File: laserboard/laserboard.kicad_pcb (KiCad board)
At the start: 4 copper layers, 167.5 x 113.5 mm, 90 parts, among them J1 Conn_01x02, J2 USB_C_Receptacle_USB2.0_16P, J3 Conn_01x19, J4 Conn_01x19, U1 AD8656, U2 PGA112, U3 AD8655, U5 NCP1117-3.3_SOT223, U6 W25Q128JVS, U7 RP2040, Y1 ABM8-272-T3

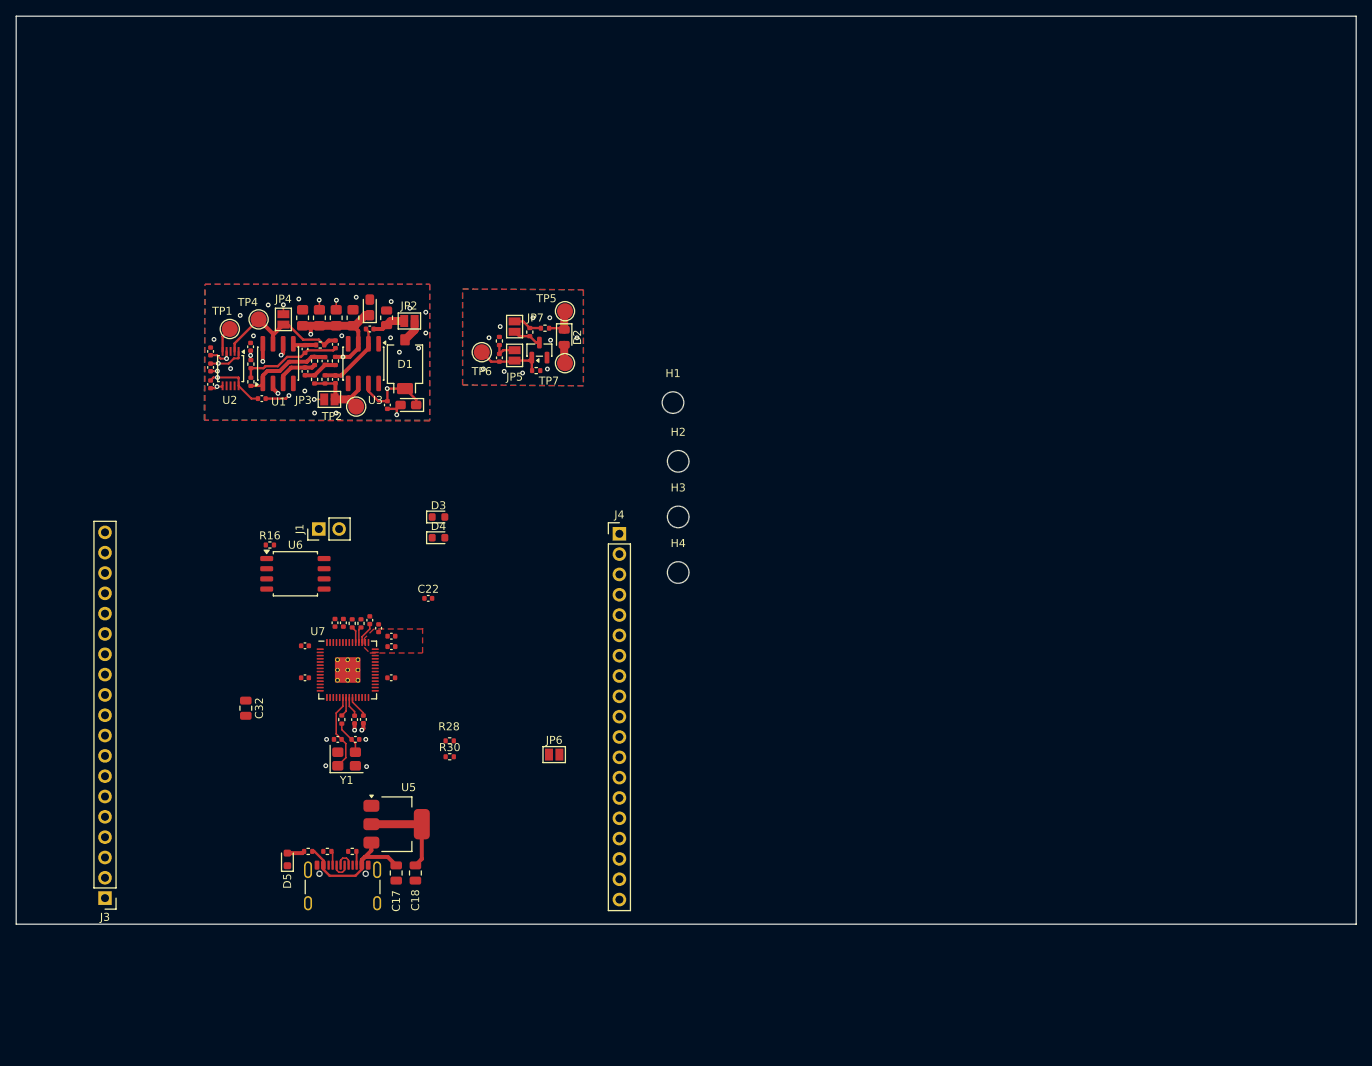
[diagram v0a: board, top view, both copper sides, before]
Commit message: PCB_prot
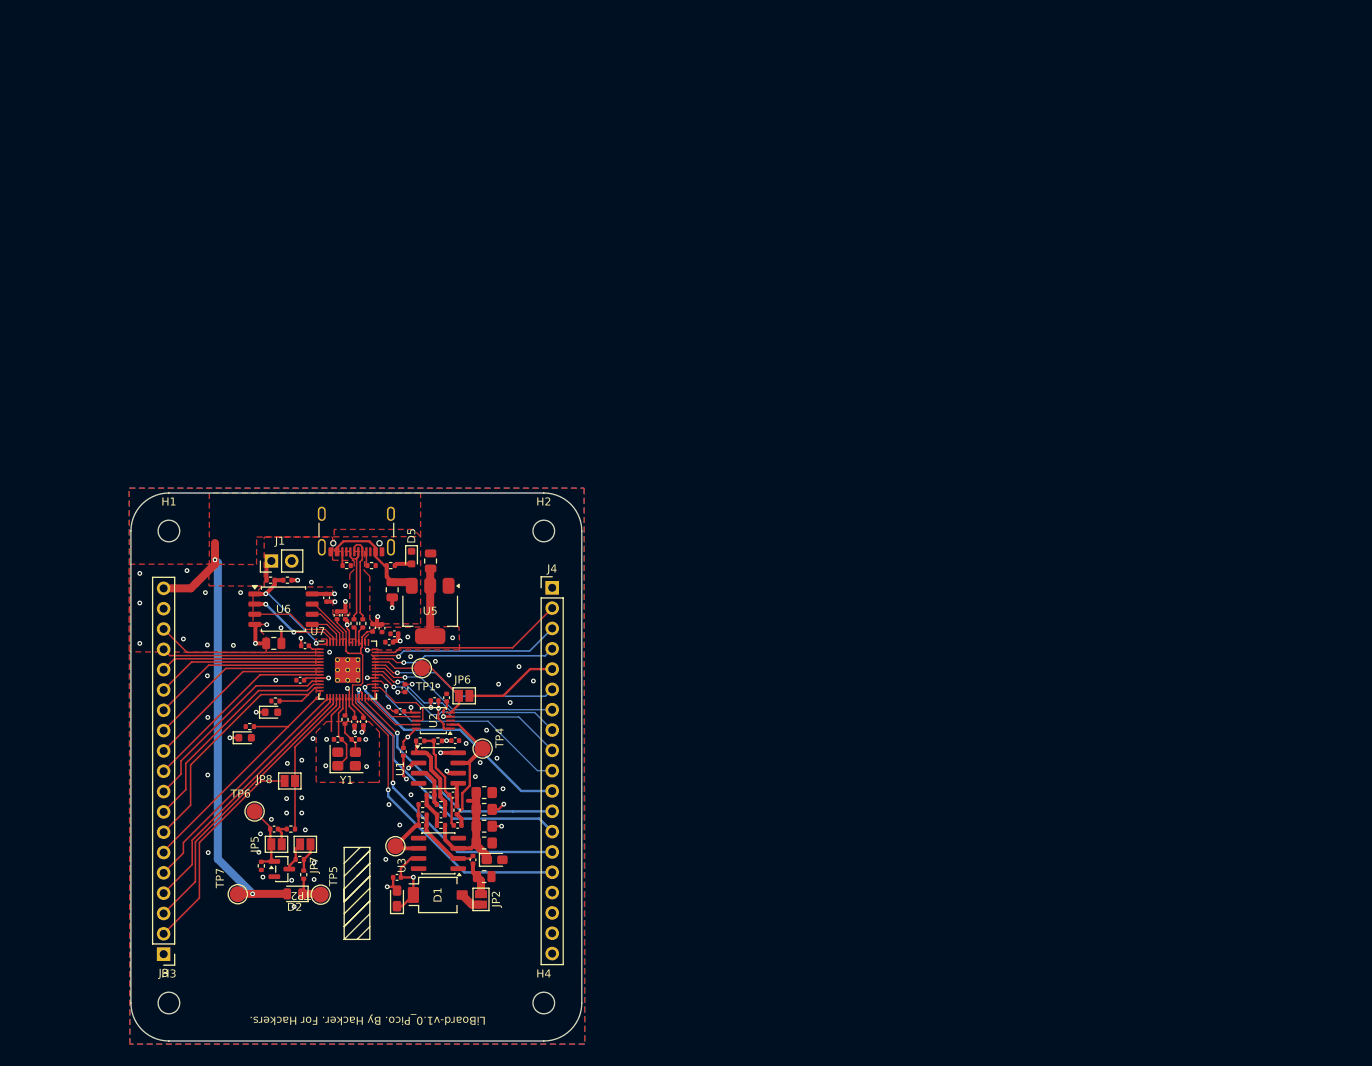
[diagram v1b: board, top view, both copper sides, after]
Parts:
- removed JP3, JP4: SolderJumper_2_Open, Jumper:SolderJumper-2_P1.3mm_Open_Pad1.0x1.5mm
- added JP8: SolderJumper_2_Open, Jumper:SolderJumper-2_P1.3mm_Open_Pad1.0x1.5mm, F.Cu at (117.2, 133.1)
- added R17: DNF, Resistor_SMD:R_0402_1005Metric, F.Cu at (116.9, 108.0)
- moved H3 88.0 mm to (102.1, 160.8)
- moved TP5 79.1 mm to (121.1, 147.3), turned to 180 degrees
- moved TP7 78.0 mm to (110.7, 147.2), turned to 180 degrees
- moved D2 77.3 mm to (117.8, 147.2), turned to 180 degrees
- moved R13 74.7 mm to (118.9, 144.8), turned to -90 degrees
- moved JP2 72.9 mm to (141.1, 147.9), turned to -90 degrees
- moved N-MOS1 72.4 mm to (116.2, 144.1), turned to 0 degrees
- moved R27 71.9 mm to (118.5, 142.9), turned to 0 degrees
- moved R29 70.9 mm to (141.5, 145.1), turned to 180 degrees
- moved R15 70.8 mm to (113.6, 143.7), turned to 90 degrees
- moved C33 70.8 mm to (142.8, 142.9), turned to 0 degrees
- moved JP7 69.8 mm to (119.1, 141.0), turned to 180 degrees
- moved JP5 68.0 mm to (115.5, 141.0), turned to 0 degrees
- moved R26 67.7 mm to (141.5, 140.8), turned to 0 degrees
- moved C20 67.6 mm to (140.1, 142.9), turned to -90 degrees
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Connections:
- J4 pad 12: /Didital/GPIO19 -> /Didital/GPIO16
- J4 pad 13: /Didital/GPIO18 -> /Didital/RUN
- J4 pad 14: /Didital/GPIO17 -> /Didital/SWD
- J4 pad 15: /Didital/GPIO16 -> /Didital/SWCLK
- J4 pad 16: /Didital/RUN -> GND
- J4 pad 17: /Didital/SWD -> GND
- J4 pad 18: /Didital/SWCLK -> GND
- R14 pad 1: /Didital/GPIO0 -> /Didital/TX_D_IN
- R28 pad 2: /Didital/GPIO25 -> /Didital/GPIO10
- R30 pad 2: /Didital/GPIO24 -> /Didital/GPIO11
- U7 pad 18: /Didital/GPIO15 -> /Didital/TX_D_IN
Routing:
- net +5V: track 19.5 -> 74.2 mm, vias 0 -> 2
- net /Didital/SWCLK: track 0.00 -> 38.5 mm, vias 0 -> 1
- net /Didital/SWD: track 0.00 -> 36.3 mm, vias 0 -> 1
- net /Didital/GPIO14: track 0.00 -> 35.8 mm
- net /Didital/RUN: track 0.00 -> 35.3 mm, vias 0 -> 1
- net /Didital/GPIO10: track 0.00 -> 33.9 mm
- net /Didital/GPIO13: track 0.00 -> 33.1 mm
- net /Didital/GPIO11: track 0.00 -> 32.6 mm
- net /Didital/GPIO16: track 0.00 -> 30.6 mm, vias 0 -> 1
- net /Didital/GPIO20: track 0.00 -> 30.4 mm, vias 0 -> 1
- net /Didital/GPIO12: track 0.00 -> 30.4 mm
- net /Didital/GPIO9: track 0.00 -> 28.1 mm
- net /Didital/GPIO21: track 0.00 -> 27.5 mm, vias 0 -> 1
- net /Didital/GPIO15: track 0.00 -> 27.1 mm
- net /Didital/GPIO22: track 0.00 -> 26.3 mm, vias 0 -> 1
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- added copper zone on F.Cu, net +5V
- removed copper zone on In2.Cu, net GND
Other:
- board size 167.5 x 113.5 mm -> 56.4 x 68.5 mm
- board text added: "LiBoard-v1.0_Pico. By Hacker. For Hackers."

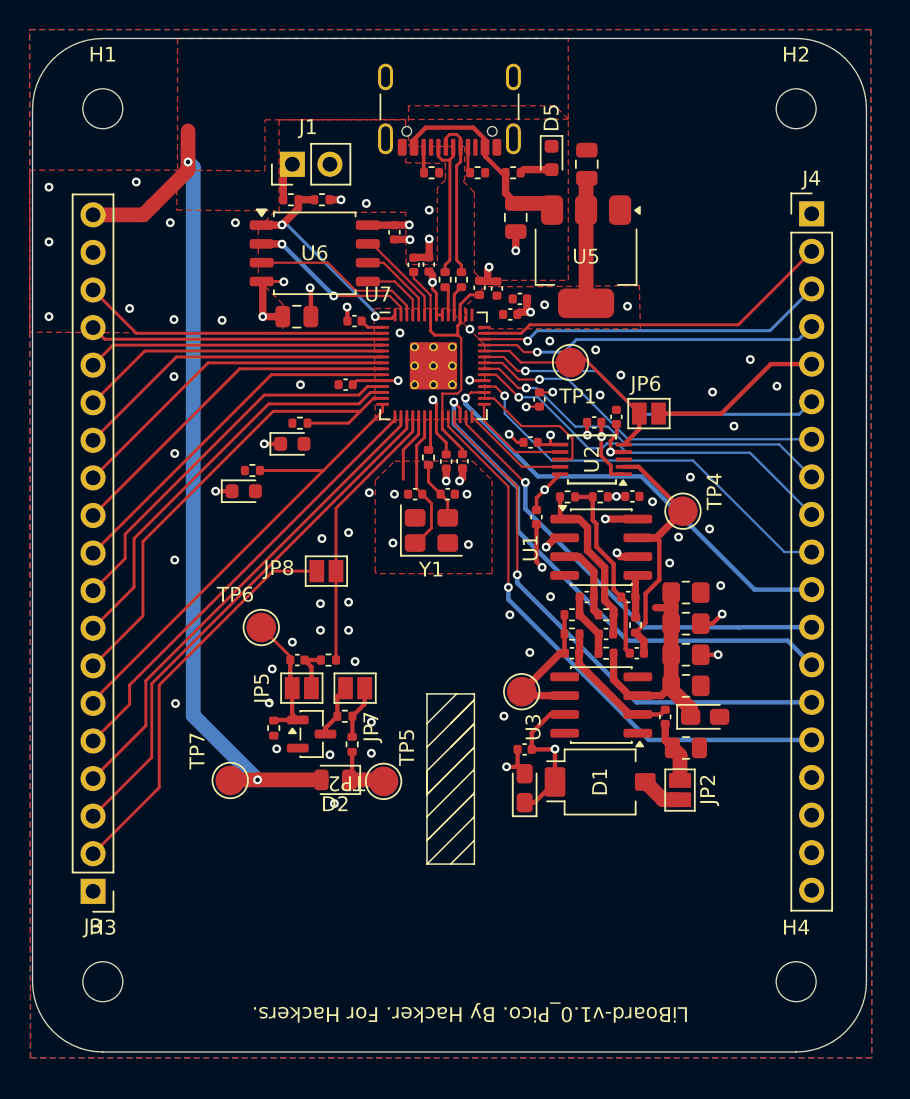
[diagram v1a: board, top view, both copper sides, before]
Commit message: PCB_done
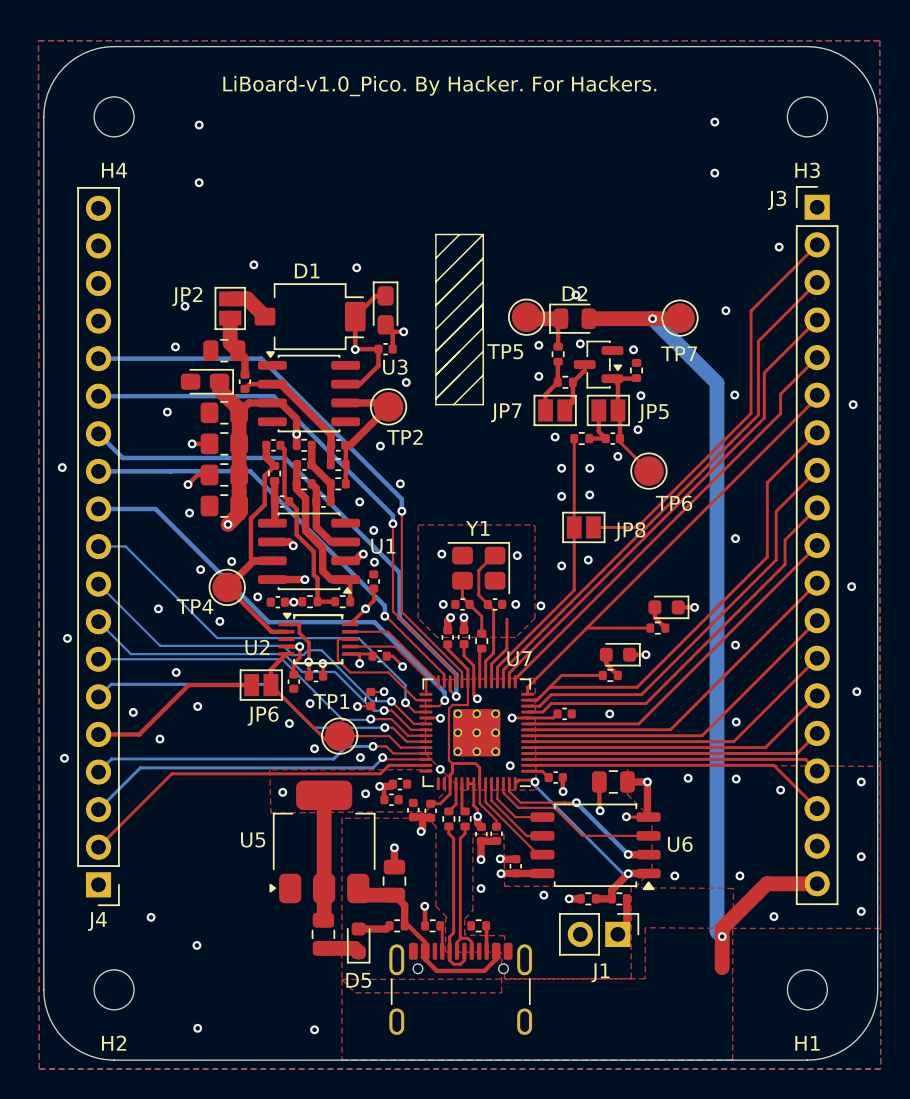
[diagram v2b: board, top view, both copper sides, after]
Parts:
- moved H1 76.2 mm to (149.7, 161.4), turned to 180 degrees
- moved H3 75.4 mm to (149.7, 102.4), turned to 180 degrees
- moved H2 75.3 mm to (102.8, 161.4), turned to 180 degrees
- moved H4 74.4 mm to (102.8, 102.4), turned to 180 degrees
- moved J3 67.3 mm to (150.4, 108.5), turned to 0 degrees
- moved J4 66.2 mm to (101.8, 154.3), turned to 180 degrees
- moved J2 61.7 mm to (126.3, 162.5), turned to 0 degrees
- moved J1 56.5 mm to (136.9, 157.7), turned to -90 degrees
- moved C18 55.0 mm to (117.0, 157.7), turned to -90 degrees
- moved D5 54.5 mm to (119.4, 158.1), turned to 90 degrees
- moved R16 52.2 mm to (137.0, 155.2), turned to 0 degrees
- moved R31 51.5 mm to (122.0, 157.1), turned to 0 degrees
- moved R22 51.0 mm to (127.5, 157.1), turned to 180 degrees
- moved R21 51.0 mm to (124.4, 157.1), turned to 180 degrees
- moved R17 50.6 mm to (134.9, 155.2), turned to 0 degrees
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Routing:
- net Net-(D3-A): track 0.14 -> 1.87 mm
- net Net-(D4-A): track 0.00 -> 1.69 mm
- net GND: track 33.6 -> 34.2 mm, vias 71 -> 94
- net /Didital/GPIO16: track 30.6 -> 30.0 mm
- net /RX frontend/Vref_Filter: track 48.4 -> 48.9 mm, vias 4 -> 6
